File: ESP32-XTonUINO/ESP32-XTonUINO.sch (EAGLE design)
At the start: 77 parts, among them CON1 MINI-USB_B5, T1 BC817

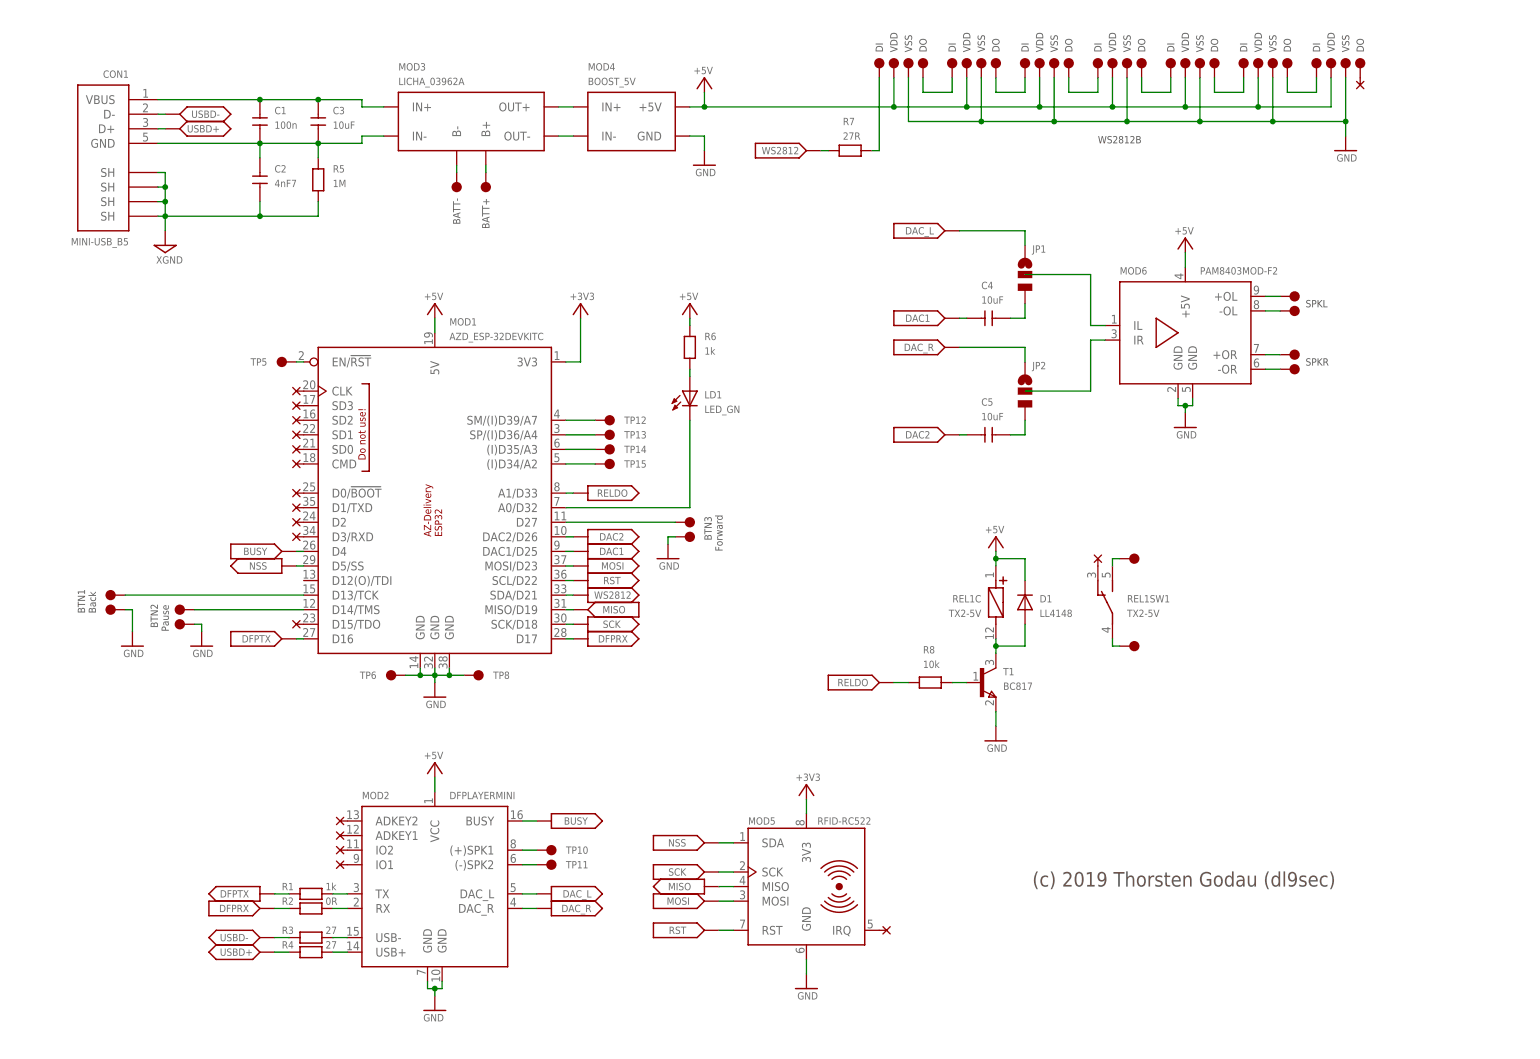
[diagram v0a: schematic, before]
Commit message: Add files via upload
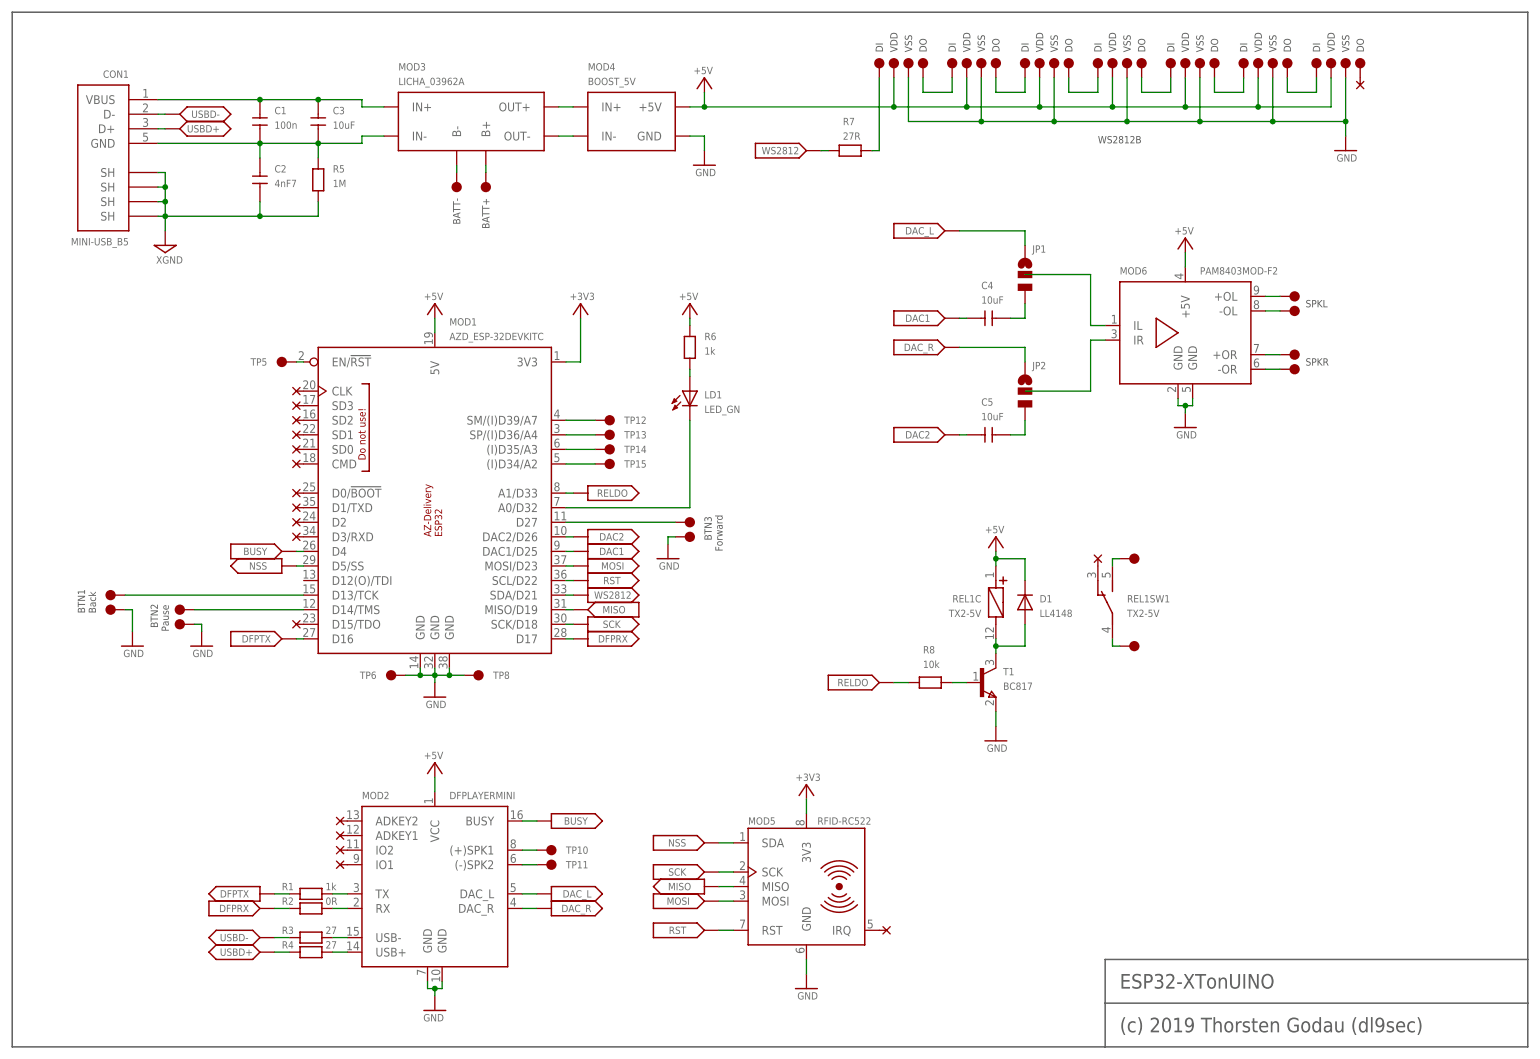
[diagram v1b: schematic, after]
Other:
- note added: "ESP32-XTonUINO"
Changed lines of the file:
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@@
 <layer number="97" name="Info" color="7" fill="1" visible="yes" active="yes"/>
 <layer number="98" name="Guide" color="6" fill="1" visible="yes" active="yes"/>
-<layer number="100" name="Logo" color="8" fill="1" visible="yes" active="yes"/>
-<layer number="101" name="Hidden" color="15" fill="1" visible="yes" active="yes"/>
-<layer number="102" name="Changes" color="12" fill="1" visible="yes" active="yes"/>
-<layer number="103" name="tMap" color="7" fill="1" visible="no" active="yes"/>
-<layer number="104" name="Name" color="7" fill="1" visible="yes" active="yes"/>
-<layer number="105" name="tPlate" color="7" fill="1" visible="no" active="yes"/>
-<layer number="106" name="bPlate" color="7" fill="1" visible="no" active="yes"/>
-<layer number="107" name="Crop" color="7" fill="1" visible="no" active="yes"/>
-<layer number="116" name="Patch_BOT" color="9" fill="4" visible="yes" active="yes"/>
-<layer number="121" name="_tsilk" color="7" fill="1" visible="yes" active="yes"/>
-<layer number="122" name="_bsilk" color="7" fill="1" visible="yes" active="yes"/>
-<layer number="125" name="_tNames" color="7" fill="1" visible="no" active="yes"/>
-<layer number="144" name="Drill_legend" color="7" fill="1" visible="no" active="yes"/>
-<layer number="151" name="tDummy" color="4" fill="1" visible="no" active="yes"/>
-<layer number="152" name="bDummy" color="1" fill="1" visible="no" active="yes"/>
-<layer number="200" name="200bmp" color="1" fill="10" visible="no" active="no"/>
-<layer number="201" name="tLogo" color="4" fill="1" visible="yes" active="yes"/>
-<layer number="202" name="202bmp" color="3" fill="1" visible="no" active="no"/>
-<layer number="203" name="203bmp" color="4" fill="10" visible="no" active="yes"/>
-<layer number="204" name="204bmp" color="5" fill="10" visible="no" active="yes"/>
-<layer number="205" name="205bmp" color="6" fill="10" visible="no" active="yes"/>
-<layer number="206" name="206bmp" color="7" fill="10" visible="no" active="yes"/>
-<layer number="207" name="207bmp" color="8" fill="10" visible="no" active="yes"/>
-<layer number="208" name="208bmp" color="9" fill="10" visible="no" active="yes"/>
-<layer number="209" name="209bmp" color="7" fill="1" visible="no" active="yes"/>
-<layer number="210" name="210bmp" color="7" fill="1" visible="no" active="yes"/>
-<layer number="211" name="211bmp" color="7" fill="1" visible="no" active="yes"/>
-<layer number="212" name="212bmp" color="7" fill="1" visible="no" active="yes"/>
-<layer number="213" name="213bmp" color="7" fill="1" visible="no" active="yes"/>
-<layer number="214" name="214bmp" color="7" fill="1" visible="no" active="yes"/>
-<layer number="215" name="215bmp" color="7" fill="1" visible="no" active="yes"/>
-<layer number="216" name="bLogo" color="1" fill="1" visible="yes" active="yes"/>
-<layer number="217" name="217bmp" color="18" fill="1" visible="no" active="no"/>
-<layer number="218" name="218bmp" color="19" fill="1" visible="no" active="no"/>
-<layer number="219" name="219bmp" color="20" fill="1" visible="no" active="no"/>
-<layer number="220" name="220bmp" color="21" fill="1" visible="no" active="no"/>
-<layer number="221" name="221bmp" color="22" fill="1" visible="no" active="no"/>
-<layer number="222" name="222bmp" color="23" fill="1" visible="no" active="no"/>
-<layer number="223" name="223bmp" color="24" fill="1" visible="no" active="no"/>
-<layer number="224" name="224bmp" color="25" fill="1" visible="no" active="no"/>
-<layer number="250" name="Descript" color="3" fill="1" visible="no" active="no"/>
-<layer number="251" name="SMDround" color="12" fill="11" visible="no" active="no"/>
-<layer number="254" name="OrgLBR" color="13" fill="1" visible="no" active="yes"/>
 </layers>
 <schematic xreflabel="%F%N/%S.%C%R" xrefpart="/%S.%C%R">
@@
 </classes>
 <parts>
-<part name="FRAME1" library="frames" deviceset="DINA4_L" device=""/>
 <part name="+5V1" library="dl9sec_public" deviceset="+5V" device=""/>
 <part name="C4" library="dl9sec_public" deviceset="C" device="0805" value="10uF"/>
@@
 <sheet>
 <plain>
-<text x="177.8" y="27.94" size="2.54" layer="97">(c) 2019 Thorsten Godau (dl9sec)</text>
+<text x="193.04" y="2.54" size="2.54" layer="97">(c) 2019 Thorsten Godau (dl9sec)</text>
 <text x="121.92" y="88.265" size="1.27" layer="97" rot="R90">BTN3</text>
 <text x="25.4" y="73.025" size="1.27" layer="97" rot="R90">BTN2</text>
@@
 <text x="76.835" y="147.955" size="1.27" layer="97" rot="R270">BATT-</text>
 <text x="81.915" y="147.955" size="1.27" layer="97" rot="R270">BATT+</text>
+<wire x1="0" y1="0" x2="190.5" y2="0" width="0.254" layer="97"/>
+<wire x1="190.5" y1="0" x2="264.16" y2="0" width="0.254" layer="97"/>
+<wire x1="264.16" y1="15.24" x2="264.16" y2="180.34" width="0.254" layer="97"/>
+<wire x1="264.16" y1="180.34" x2="0" y2="180.34" width="0.254" layer="97"/>
+<wire x1="0" y1="180.34" x2="0" y2="0" width="0.254" layer="97"/>
+<wire x1="190.5" y1="0" x2="190.5" y2="7.62" width="0.254" layer="97"/>
+<wire x1="190.5" y1="7.62" x2="190.5" y2="15.24" width="0.254" layer="97"/>
+<wire x1="190.5" y1="15.24" x2="264.16" y2="15.24" width="0.254" layer="97"/>
+<wire x1="264.16" y1="15.24" x2="264.16" y2="7.62" width="0.254" layer="97"/>
+<wire x1="264.16" y1="7.62" x2="264.16" y2="0" width="0.254" layer="97"/>
+<wire x1="190.5" y1="7.62" x2="264.16" y2="7.62" width="0.254" layer="97"/>
+<text x="193.04" y="10.16" size="2.54" layer="97">ESP32-XTonUINO</text>
 </plain>
 <instances>
-<instance part="FRAME1" gate="G$1" x="0" y="0"/>
-<instance part="FRAME1" gate="G$2" x="162.56" y="0"/>
 <instance part="+5V1" gate="G$1" x="73.66" y="127"/>
 <instance part="C4" gate="G$1" x="166.37" y="127" smashed="yes">
